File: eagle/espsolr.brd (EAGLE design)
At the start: 70.8 x 44.4 mm, 17 parts, among them IC1 ATtiny85

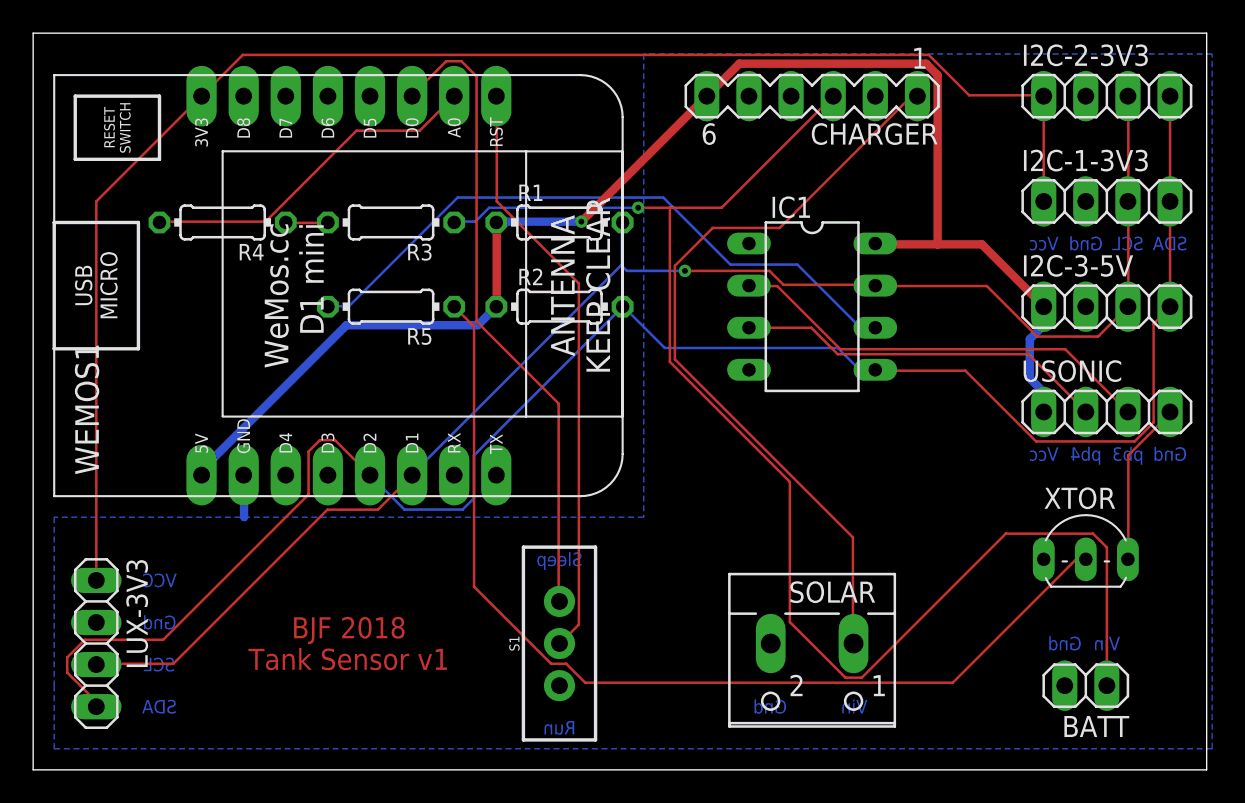
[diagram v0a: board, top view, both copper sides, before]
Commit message: tweaked size and layers
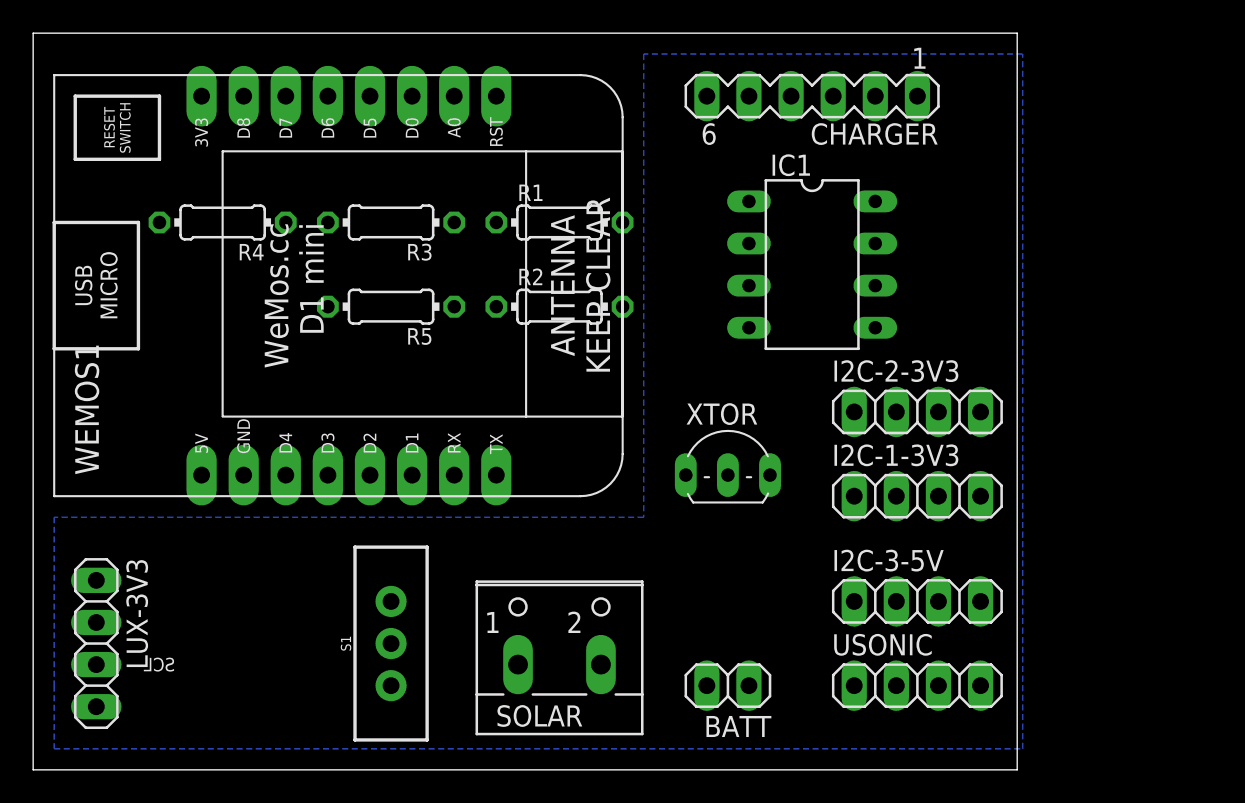
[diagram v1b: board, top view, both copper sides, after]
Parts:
- moved I2C-2-3V3 22.2 mm to (53.3, 21.6)
- moved XTOR 22.2 mm to (41.9, 19.1)
- moved BATT 21.6 mm to (41.9, 5.08)
- moved I2C-1-3V3 21.1 mm to (53.3, 16.5)
- moved I2C-3-5V 21.1 mm to (53.3, 10.2)
- moved USONIC 20.1 mm to (53.3, 5.08)
- moved SOLAR 15.3 mm to (31.8, 7.62), turned to 0 degrees
- moved S1 10.2 mm to (21.6, 7.62)
- moved IC1 2.54 mm to (47.0, 30.5)
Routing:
- net SDA: track 108.5 -> 0.00 mm
- net +3V3: track 91.1 -> 0.00 mm
- net SCL: track 90.2 -> 0.00 mm, vias 1 -> 0
- net +5V: track 87.2 -> 0.00 mm, vias 1 -> 0
- net BAT+: track 86.8 -> 0.00 mm, vias 1 -> 0
- net N$10: track 59.8 -> 0.00 mm
- net SOLAR+: track 46.2 -> 0.00 mm
- net NPN: track 39.0 -> 0.00 mm
- net D0: track 38.9 -> 0.00 mm
- net RESET: track 35.6 -> 0.00 mm
- net N$7: track 26.0 -> 0.00 mm
- net N$8: track 22.4 -> 0.00 mm
- net N$2: track 21.0 -> 0.00 mm
- net N$9: track 9.94 -> 0.00 mm
- net N$1: track 2.58 -> 0.00 mm
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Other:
- board size 70.8 x 44.4 mm -> 59.4 x 44.4 mm
- board text added: "BJF 2018 Tank Sensor v1.1"
- board text removed: "BJF 2018 Tank Sensor v1"
